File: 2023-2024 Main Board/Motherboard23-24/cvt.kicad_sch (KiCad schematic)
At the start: 0 parts

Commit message: Close to finishing up 2023-2024 Main Board Schematic
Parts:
- added J1: Conn_01x06_Pin, symbol Connector:Conn_01x06_Pin
- added J18: Conn_01x02_Pin, symbol Connector:Conn_01x02_Pin
- added J19, J7: Conn_01x03_Pin, symbol Connector:Conn_01x03_Pin
- added U1: ARDUINO_PRO_MINI, ARDUINO_PRO_MINI:MODULE_ARDUINO_PRO_MINI, symbol ARDUINO_PRO_MINI:ARDUINO_PRO_MINI
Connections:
- new net: J18.1 (Pin_1), U1.JP7_5 (D5)
- new net: J18.2 (Pin_2), U1.JP7_6 (D4)
- new net: J7.1 (Pin_1), U1.JP7_7 (D3)
- new net: J7.2 (Pin_2), U1.JP7_8 (D2)
- new net: J1.1 (Pin_1), U1.JP1_1 (DTR)
- new net: J1.2 (Pin_2), U1.JP1_2 (TXO)
- new net: J1.3 (Pin_3), U1.JP1_3 (RXI)
- new net: J1.5 (Pin_5), J1.6 (Pin_6), U1.JP1_5 (GND), U1.JP1_6 (GND)
- new net +5V: J7.3 (Pin_3), U1.JP6_4 (VCC_1)
- new net GND: U1.JP6_2 (GND_1), U1.JP7_9 (GND_2)
- no-connect marks 0 -> 1
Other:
- note added: "CVT Actuator Inputs"
- note added: "CVT Controls"
- note added: "CVT Inputs"
- note added: "DTR"
- note added: "GND"
- note added: "In"
- note added: "Out"
- note added: "Programming pins"
- note added: "RXI"
- note added: "TX0"

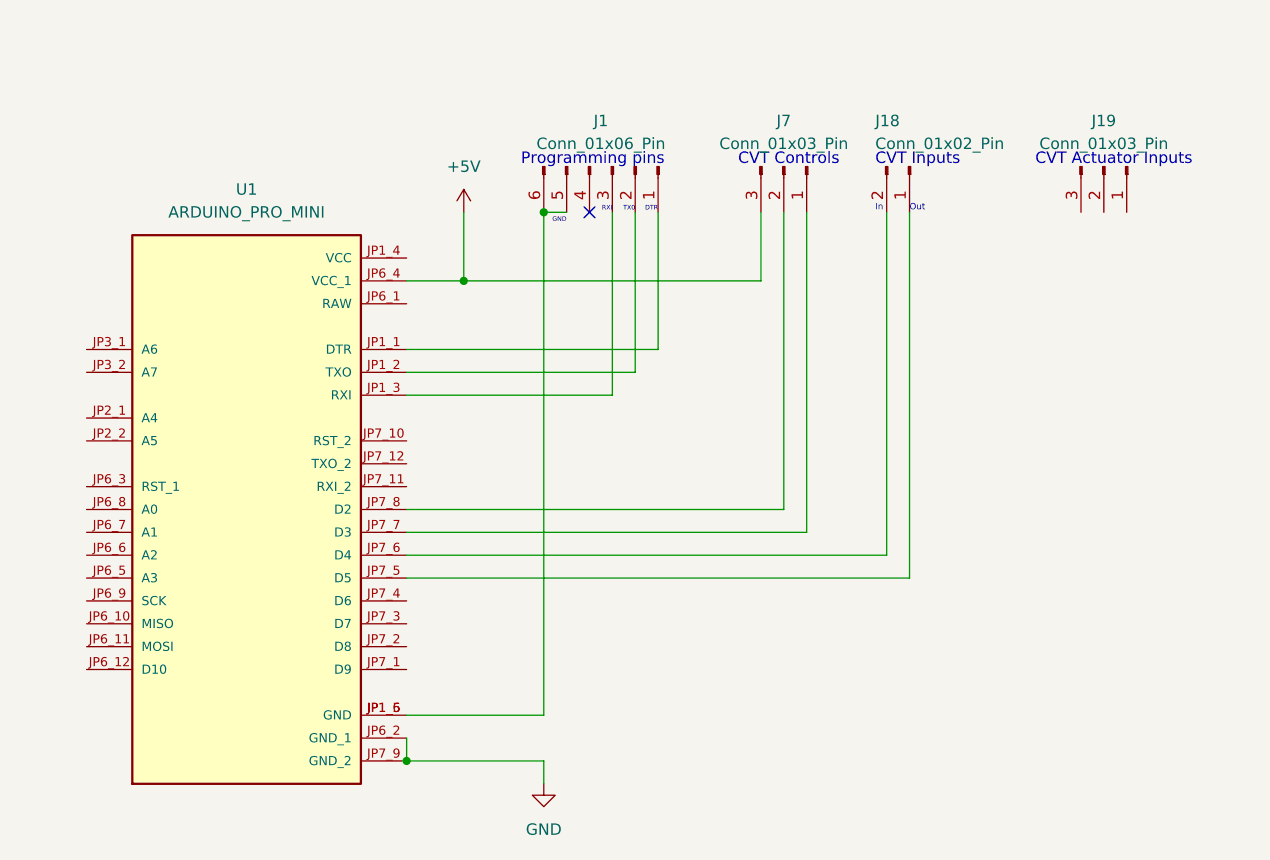
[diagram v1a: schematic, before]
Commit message: first draft of 23-24 Main Board
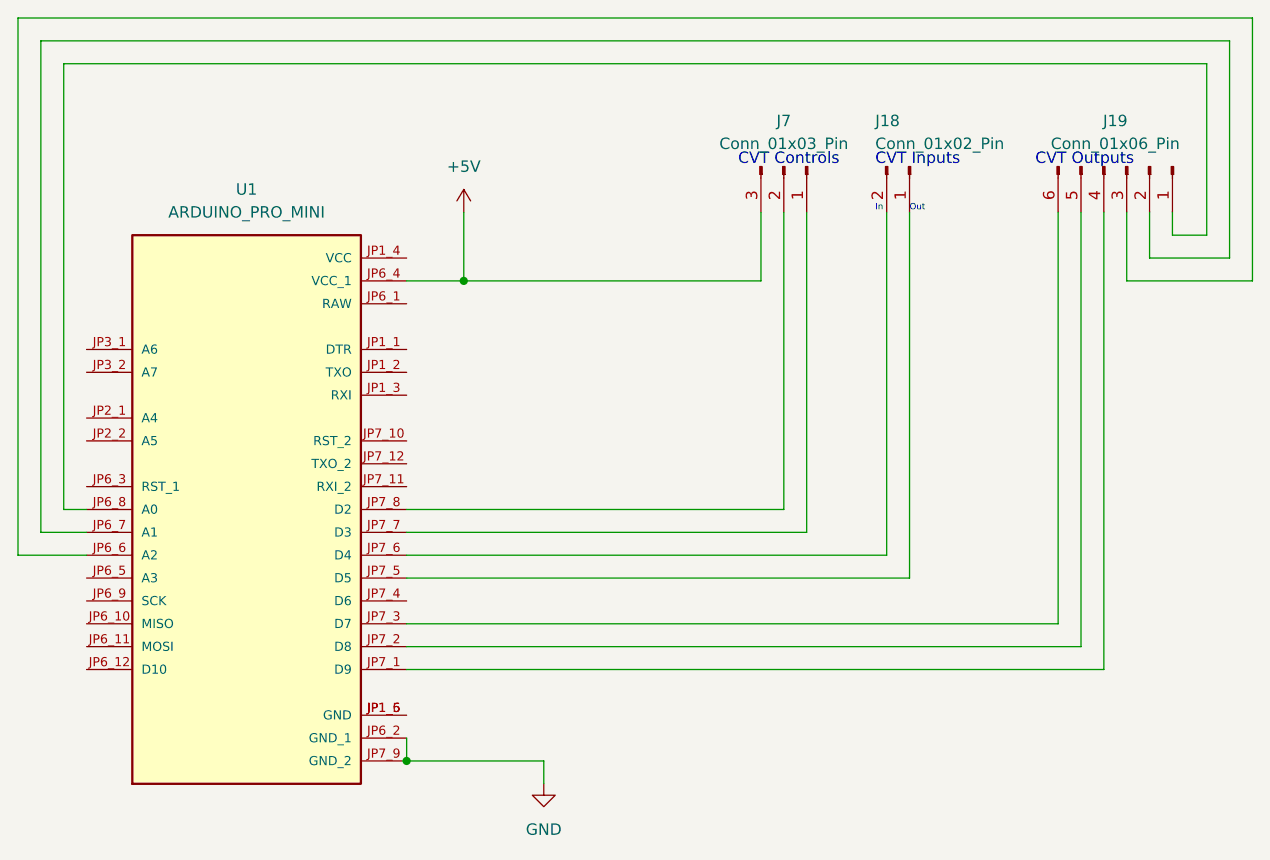
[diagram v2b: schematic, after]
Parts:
- removed J1: Conn_01x06_Pin, symbol Connector:Conn_01x06_Pin
- removed J19: Conn_01x03_Pin, symbol Connector:Conn_01x03_Pin
- added J19: Conn_01x06_Pin, TerminalBlock_Phoenix:TerminalBlock_Phoenix_MKDS-1,5-6-5.08_1x06_P5.08mm_Horizontal, symbol Connector:Conn_01x06_Pin
- J18: footprint (none) -> TerminalBlock_Phoenix:TerminalBlock_Phoenix_MKDS-1,5-2-5.08_1x02_P5.08mm_Horizontal
- J7: footprint (none) -> TerminalBlock_Phoenix:TerminalBlock_Phoenix_MKDS-3-3-5.08_1x03_P5.08mm_Horizontal
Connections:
- net at U1.JP6_6 (A2): now also J19.3 (Pin_3)
- net at U1.JP6_7 (A1): now also J19.2 (Pin_2)
- net at U1.JP6_8 (A0): now also J19.1 (Pin_1)
- net at U1.JP7_1 (D9): now also J19.4 (Pin_4)
- net at U1.JP7_2 (D8): now also J19.5 (Pin_5)
- net at U1.JP7_3 (D7): now also J19.6 (Pin_6)
- no-connect marks 1 -> 0
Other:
- note added: "CVT Outputs"
- note removed: "CVT Actuator Inputs"
- note removed: "DTR"
- note removed: "GND"
- note removed: "Programming pins"
- note removed: "RXI"
- note removed: "TX0"
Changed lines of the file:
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@@
   (junction (at 120.65 69.85) (diameter 0) (color 0 0 0 0)
   )
-  (junction (at 129.54 62.23) (diameter 0) (color 0 0 0 0)
-  )
-  (no_connect (at 134.62 62.23))
   (wire (pts (xy 156.21 95.25) (xy 156.21 62.23))
     (stroke (width 0) (type default))
   )
+  (wire (pts (xy 196.85 62.23) (xy 196.85 67.31))
+    (stroke (width 0) (type default))
+  )
+  (wire (pts (xy 199.39 64.77) (xy 203.2 64.77))
+    (stroke (width 0) (type default))
+  )
   (wire (pts (xy 170.18 102.87) (xy 170.18 62.23))
     (stroke (width 0) (type default))
   )
-  (wire (pts (xy 129.54 62.23) (xy 129.54 118.11))
-    (stroke (width 0) (type default))
-  )
-  (wire (pts (xy 114.3 80.01) (xy 139.7 80.01))
-    (stroke (width 0) (type default))
-  )
-  (wire (pts (xy 129.54 62.23) (xy 132.08 62.23))
+  (wire (pts (xy 191.77 113.03) (xy 114.3 113.03))
+    (stroke (width 0) (type default))
+  )
+  (wire (pts (xy 73.66 43.18) (xy 205.74 43.18))
+    (stroke (width 0) (type default))
+  )
+  (wire (pts (xy 189.23 110.49) (xy 114.3 110.49))
+    (stroke (width 0) (type default))
+  )
+  (wire (pts (xy 196.85 67.31) (xy 205.74 67.31))
+    (stroke (width 0) (type default))
+  )
+  (wire (pts (xy 76.2 45.72) (xy 76.2 95.25))
+    (stroke (width 0) (type default))
+  )
+  (wire (pts (xy 191.77 62.23) (xy 191.77 113.03))
+    (stroke (width 0) (type default))
+  )
+  (wire (pts (xy 76.2 45.72) (xy 203.2 45.72))
     (stroke (width 0) (type default))
   )
@@
     (stroke (width 0) (type default))
   )
-  (wire (pts (xy 114.3 77.47) (xy 142.24 77.47))
-    (stroke (width 0) (type default))
-  )
-  (wire (pts (xy 114.3 82.55) (xy 137.16 82.55))
-    (stroke (width 0) (type default))
-  )
   (wire (pts (xy 120.65 69.85) (xy 153.67 69.85))
     (stroke (width 0) (type default))
   )
-  (wire (pts (xy 139.7 62.23) (xy 139.7 80.01))
+  (wire (pts (xy 71.12 100.33) (xy 78.74 100.33))
     (stroke (width 0) (type default))
   )
@@
     (stroke (width 0) (type default))
   )
-  (wire (pts (xy 142.24 62.23) (xy 142.24 77.47))
+  (wire (pts (xy 71.12 40.64) (xy 208.28 40.64))
     (stroke (width 0) (type default))
   )
@@
     (stroke (width 0) (type default))
   )
-  (wire (pts (xy 129.54 118.11) (xy 114.3 118.11))
+  (wire (pts (xy 194.31 62.23) (xy 194.31 69.85))
+    (stroke (width 0) (type default))
+  )
+  (wire (pts (xy 205.74 67.31) (xy 205.74 43.18))
     (stroke (width 0) (type default))
   )
@@
     (stroke (width 0) (type default))
   )
-  (wire (pts (xy 137.16 62.23) (xy 137.16 82.55))
-    (stroke (width 0) (type default))
-  )
   (wire (pts (xy 158.75 62.23) (xy 158.75 97.79))
     (stroke (width 0) (type default))
   )
+  (wire (pts (xy 73.66 43.18) (xy 73.66 97.79))
+    (stroke (width 0) (type default))
+  )
+  (wire (pts (xy 199.39 62.23) (xy 199.39 64.77))
+    (stroke (width 0) (type default))
+  )
+  (wire (pts (xy 194.31 69.85) (xy 208.28 69.85))
+    (stroke (width 0) (type default))
+  )
+  (wire (pts (xy 73.66 97.79) (xy 78.74 97.79))
+    (stroke (width 0) (type default))
+  )
+  (wire (pts (xy 189.23 62.23) (xy 189.23 110.49))
+    (stroke (width 0) (type default))
+  )
+  (wire (pts (xy 208.28 69.85) (xy 208.28 40.64))
+    (stroke (width 0) (type default))
+  )
   (wire (pts (xy 114.3 95.25) (xy 156.21 95.25))
     (stroke (width 0) (type default))
@@
     (stroke (width 0) (type default))
   )
+  (wire (pts (xy 71.12 40.64) (xy 71.12 100.33))
+    (stroke (width 0) (type default))
+  )
+  (wire (pts (xy 186.69 107.95) (xy 114.3 107.95))
+    (stroke (width 0) (type default))
+  )
+  (wire (pts (xy 76.2 95.25) (xy 78.74 95.25))
+    (stroke (width 0) (type default))
+  )
+  (wire (pts (xy 203.2 64.77) (xy 203.2 45.72))
+    (stroke (width 0) (type default))
+  )
   (wire (pts (xy 129.54 123.19) (xy 129.54 125.73))
     (stroke (width 0) (type default))
   )
+  (wire (pts (xy 186.69 62.23) (xy 186.69 107.95))
+    (stroke (width 0) (type default))
+  )
   (wire (pts (xy 153.67 69.85) (xy 153.67 62.23))
     (stroke (width 0) (type default))
-  )
-  (text "Programming pins " (at 127 57.15 0)
-    (effects (font (size 1.27 1.27)) (justify left bottom))
-  )
-  (text "DTR" (at 142.24 62.23 0)
-    (effects (font (size 0.508 0.508)) (justify right bottom))
-  )
-  (text "GND" (at 132.08 63.5 0)
-    (effects (font (size 0.508 0.508)) (justify right bottom))
-  )
-  (text "TX0" (at 139.7 62.23 0)
-    (effects (font (size 0.508 0.508)) (justify right bottom))
   )
   (text "Out" (at 170.18 62.23 0)
@@
     (effects (font (size 1.27 1.27)) (justify left bottom))
   )
+  (text "CVT Outputs\n" (at 184.15 57.15 0)
+    (effects (font (size 1.27 1.27)) (justify left bottom))
+  )
   (text "In" (at 166.37 62.23 0)
     (effects (font (size 0.7 0.7)) (justify left bottom))
-  )
-  (text "CVT Actuator Inputs" (at 184.15 57.15 0)
-    (effects (font (size 1.27 1.27)) (justify left bottom))
-  )
-  (text "RXI" (at 137.16 62.23 0)
-    (effects (font (size 0.508 0.508)) (justify right bottom))
   )
   (text "CVT Inputs" (at 166.37 57.15 0)
@@
       (effects (font (size 1.27 1.27)) (justify left))
     )
-    (property "Footprint" "" (at 170.18 57.15 0)
+    (property "Footprint" "TerminalBlock_Phoenix:TerminalBlock_Phoenix_MKDS-1,5-2-5.08_1x02_P5.08mm_Horizontal" (at 170.18 57.15 0)
       (effects (font (size 1.27 1.27)) hide)
     )
@@
     )
   )
-  (symbol (lib_id "Connector:Conn_01x03_Pin") (at 191.77 57.15 270) (unit 1)
-    (in_bom yes) (on_board yes) (dnp no) (fields_autoplaced)
-    (property "Reference" "J19" (at 191.77 52.07 90)
-      (effects (font (size 1.27 1.27)))
-    )
-    (property "Value" "Conn_01x03_Pin" (at 191.77 54.61 90)
-      (effects (font (size 1.27 1.27)))
-    )
-    (property "Footprint" "" (at 191.77 57.15 0)
-      (effects (font (size 1.27 1.27)) hide)
-    )
-    (property "Datasheet" "~" (at 191.77 57.15 0)
+  (symbol (lib_id "Connector:Conn_01x06_Pin") (at 194.31 57.15 270) (unit 1)
+    (in_bom yes) (on_board yes) (dnp no) (fields_autoplaced)
+    (property "Reference" "J19" (at 193.04 52.07 90)
+      (effects (font (size 1.27 1.27)))
+    )
+    (property "Value" "Conn_01x06_Pin" (at 193.04 54.61 90)
+      (effects (font (size 1.27 1.27)))
+    )
+    (property "Footprint" "TerminalBlock_Phoenix:TerminalBlock_Phoenix_MKDS-1,5-6-5.08_1x06_P5.08mm_Horizontal" (at 194.31 57.15 0)
+      (effects (font (size 1.27 1.27)) hide)
+    )
+    (property "Datasheet" "~" (at 194.31 57.15 0)
       (effects (font (size 1.27 1.27)) hide)
     )
@@
     (pin "2")
     (pin "3")
+    (pin "4")
+    (pin "5")
+    (pin "6")
     (instances
       (project "Motherboard23-24"
@@
         )
         (path "/418d1727-08ff-41e8-954f-e6e13e4fb4ca/d15f88a3-eb3a-4abd-b913-7ade9bdcdd4a"
-          (reference "J25") (unit 1)
+          (reference "J1") (unit 1)
         )
       )
@@
       (effects (font (size 1.27 1.27)))
     )
-    (property "Footprint" "" (at 156.21 57.15 0)
+    (property "Footprint" "TerminalBlock_Phoenix:TerminalBlock_Phoenix_MKDS-3-3-5.08_1x03_P5.08mm_Horizontal" (at 156.21 57.15 0)
       (effects (font (size 1.27 1.27)) hide)
     )
@@
         )
       )
-    )
-  )
-  (symbol (lib_id "Connector:Conn_01x06_Pin") (at 137.16 57.15 270) (unit 1)
-    (in_bom yes) (on_board yes) (dnp no) (fields_autoplaced)
-    (property "Reference" "J1" (at 135.89 52.07 90)
-      (effects (font (size 1.27 1.27)))
-    )
-    (property "Value" "Conn_01x06_Pin" (at 135.89 54.61 90)
-      (effects (font (size 1.27 1.27)))
-    )
-    (property "Footprint" "" (at 137.16 57.15 0)
-      (effects (font (size 1.27 1.27)) hide)
-    )
-    (property "Datasheet" "~" (at 137.16 57.15 0)
-      (effects (font (size 1.27 1.27)) hide)
-    )
-    (pin "1")
-    (pin "2")
-    (pin "3")
-    (pin "4")
-    (pin "5")
-    (pin "6")
-    (instances
-      (project "Motherboard23-24"
-        (path "/418d1727-08ff-41e8-954f-e6e13e4fb4ca/97542c42-a706-445d-a930-fc308481bbac"
-          (reference "J1") (unit 1)
-        )
-        (path "/418d1727-08ff-41e8-954f-e6e13e4fb4ca/d15f88a3-eb3a-4abd-b913-7ade9bdcdd4a"
-          (reference "J22") (unit 1)
-        )
-      )
